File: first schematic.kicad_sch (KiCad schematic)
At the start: 1 part

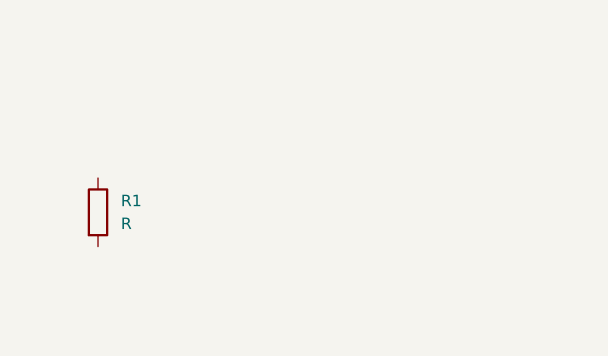
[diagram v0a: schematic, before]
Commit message: Autosave
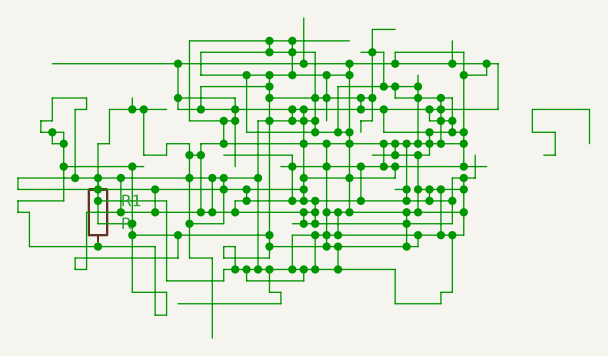
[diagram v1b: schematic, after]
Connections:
- net at R1.1: now also R1.2

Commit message: Autosave
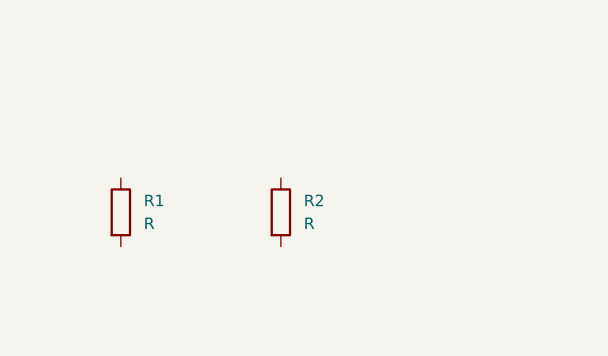
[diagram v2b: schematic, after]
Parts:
- added R2: R, symbol Device:R
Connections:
- net at R1.1: no longer R1.2
